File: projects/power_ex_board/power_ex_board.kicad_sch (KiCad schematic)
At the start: 7 parts, among them J1 USB_C_Receptacle_USB2.0, J2 3V3, J3 GND, J4 5V, J5 GND, J6 Custom, J7 GND

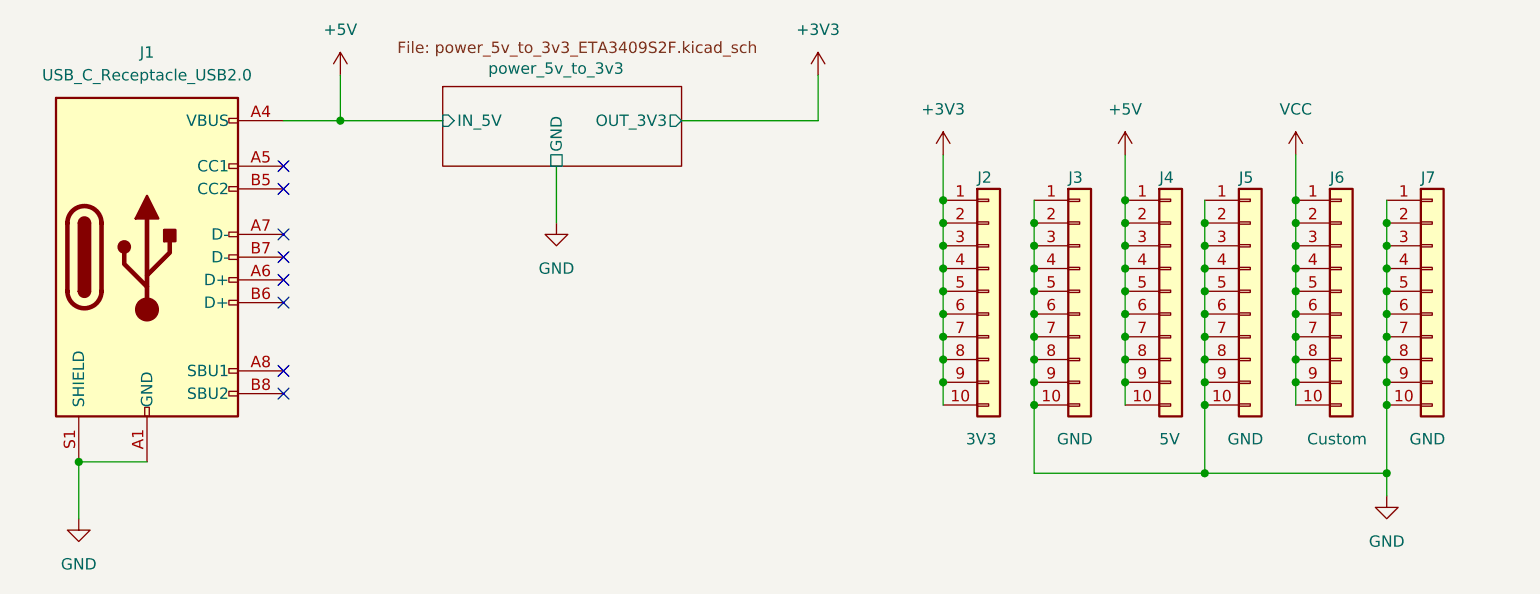
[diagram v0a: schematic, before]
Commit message: projects: add power_ex_board
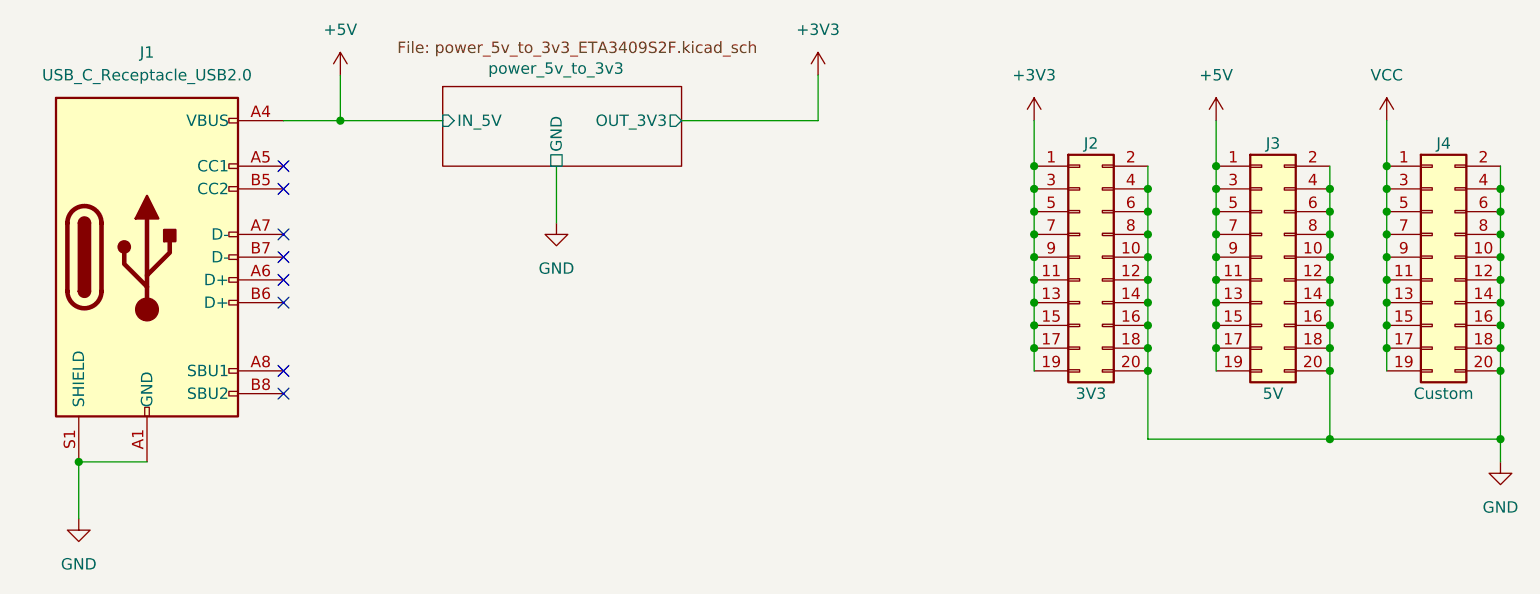
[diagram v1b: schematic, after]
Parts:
- removed J2: 3V3, Connector_PinHeader_2.54mm:PinHeader_1x10_P2.54mm_Vertical, symbol Connector_Generic:Conn_01x10
- removed J3, J5, J7: GND, Connector_PinHeader_2.54mm:PinHeader_1x10_P2.54mm_Vertical, symbol Connector_Generic:Conn_01x10
- removed J4: 5V, Connector_PinHeader_2.54mm:PinHeader_1x10_P2.54mm_Vertical, symbol Connector_Generic:Conn_01x10
- removed J6: Custom, Connector_PinHeader_2.54mm:PinHeader_1x10_P2.54mm_Vertical, symbol Connector_Generic:Conn_01x10
- added J2: 3V3, Connector_PinHeader_2.54mm:PinHeader_2x10_P2.54mm_Vertical, symbol Connector_Generic:Conn_02x10_Odd_Even
- added J3: 5V, Connector_PinHeader_2.54mm:PinHeader_2x10_P2.54mm_Vertical, symbol Connector_Generic:Conn_02x10_Odd_Even
- added J4: Custom, Connector_PinHeader_2.54mm:PinHeader_2x10_P2.54mm_Vertical, symbol Connector_Generic:Conn_02x10_Odd_Even
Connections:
- net +3V3: now also J2.1 (Pin_1), J2.11 (Pin_11), J2.13 (Pin_13), J2.15 (Pin_15), J2.17 (Pin_17), J2.19 (Pin_19), J2.3 (Pin_3), J2.5 (Pin_5), J2.7 (Pin_7), J2.9 (Pin_9)
- net +5V: now also J3.1 (Pin_1), J3.11 (Pin_11), J3.13 (Pin_13), J3.15 (Pin_15), J3.17 (Pin_17), J3.19 (Pin_19), J3.3 (Pin_3), J3.5 (Pin_5), J3.7 (Pin_7), J3.9 (Pin_9)
- net GND: now also J2.10 (Pin_10), J2.12 (Pin_12), J2.14 (Pin_14), J2.16 (Pin_16), J2.18 (Pin_18), J2.2 (Pin_2), J2.20 (Pin_20), J2.4 (Pin_4), J2.6 (Pin_6), J2.8 (Pin_8), J3.10 (Pin_10), J3.12 (Pin_12), J3.14 (Pin_14), J3.16 (Pin_16), J3.18 (Pin_18), J3.2 (Pin_2), J3.20 (Pin_20), J3.4 (Pin_4), J3.6 (Pin_6), J3.8 (Pin_8), J4.10 (Pin_10), J4.12 (Pin_12), J4.14 (Pin_14), J4.16 (Pin_16), J4.18 (Pin_18), J4.2 (Pin_2), J4.20 (Pin_20), J4.4 (Pin_4), J4.6 (Pin_6), J4.8 (Pin_8)
- net VCC: now also J4.1 (Pin_1), J4.11 (Pin_11), J4.13 (Pin_13), J4.15 (Pin_15), J4.17 (Pin_17), J4.19 (Pin_19), J4.3 (Pin_3), J4.5 (Pin_5), J4.7 (Pin_7), J4.9 (Pin_9)
